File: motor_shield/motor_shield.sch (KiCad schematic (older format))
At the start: 23 parts, among them J1 MOTOR PWR, J2 Conn_01x04, J3 Conn_01x04, J4 Conn_01x04, J5 ARDUINO PWR, J6 RPI PWR, J7 Raspberry_Pi_2_3, U1 DRV8834_CARRIER, U10 SHARP_GP2Y0A21YK0F, U2 DRV8834_CARRIER, U3 DRV8834_CARRIER, U4 ARDUINO_MICRO, U5 SHARP_GP2Y0A21YK0F, U6 SHARP_GP2Y0A21YK0F, U7 SHARP_GP2Y0A21YK0F, U8 SHARP_GP2Y0A21YK0F, U9 SHARP_GP2Y0A21YK0F

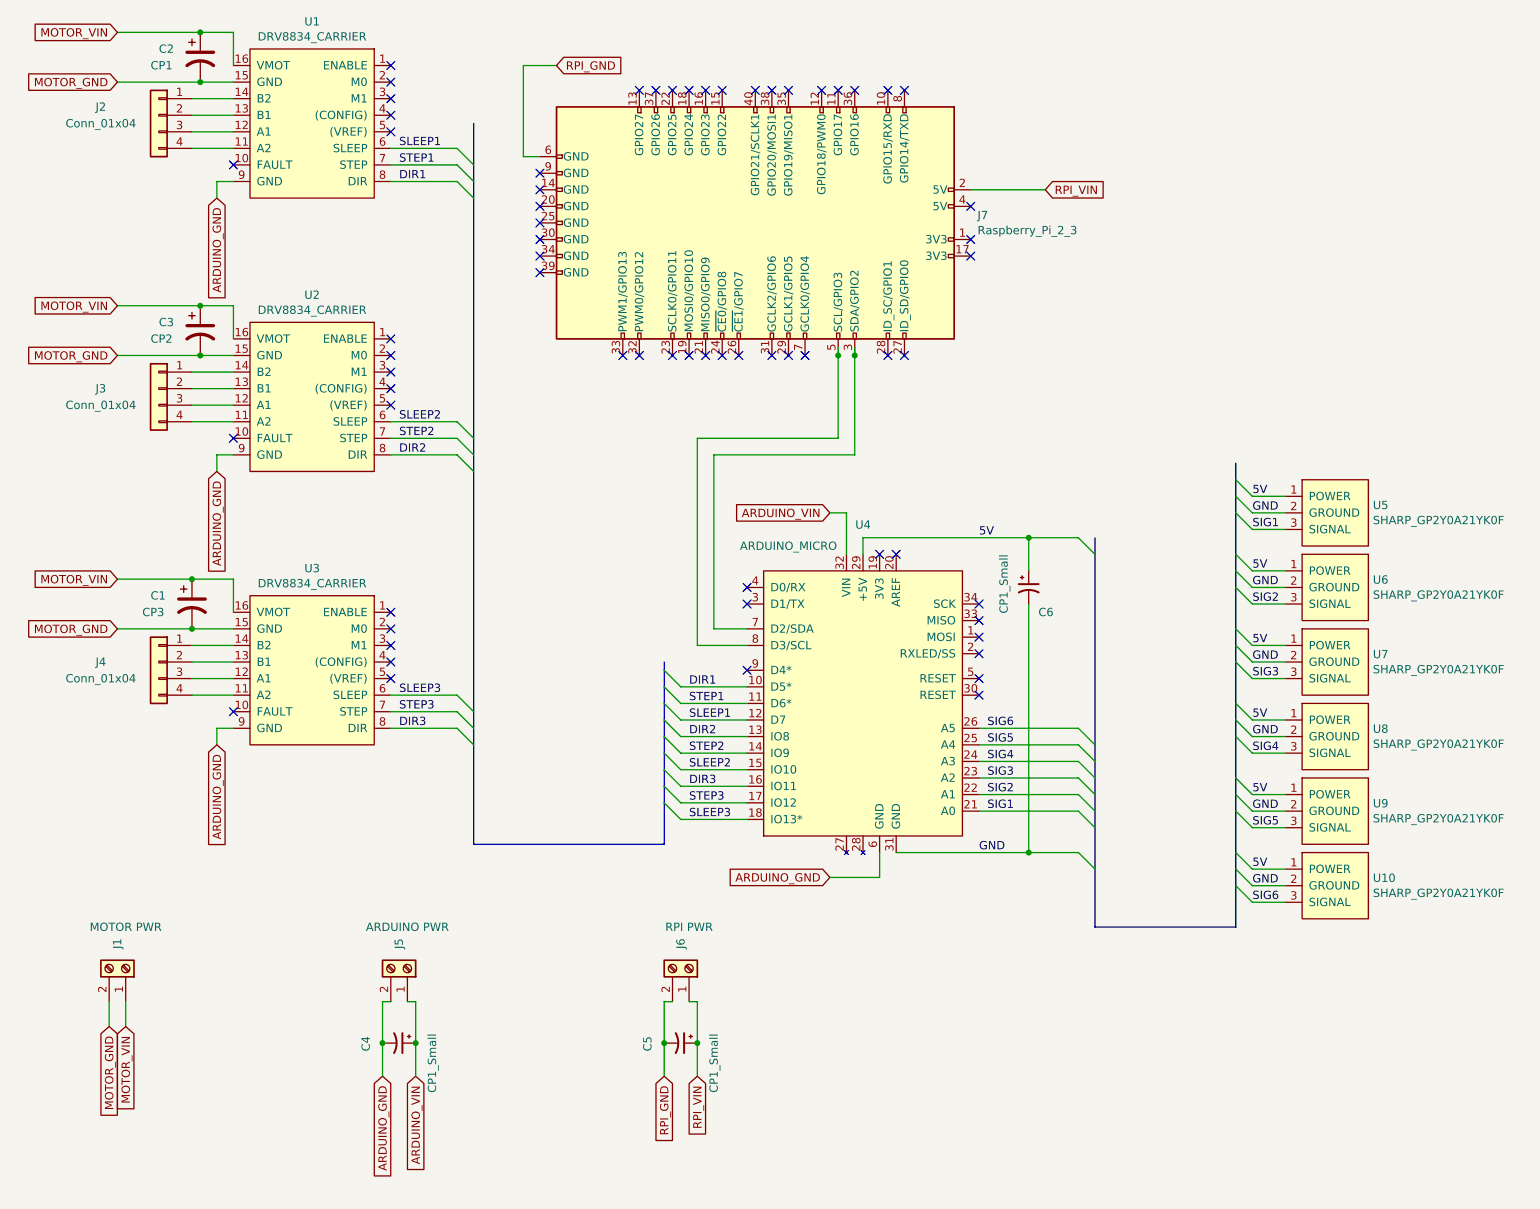
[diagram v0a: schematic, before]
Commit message: Finish circuit board design
off to oshpark!
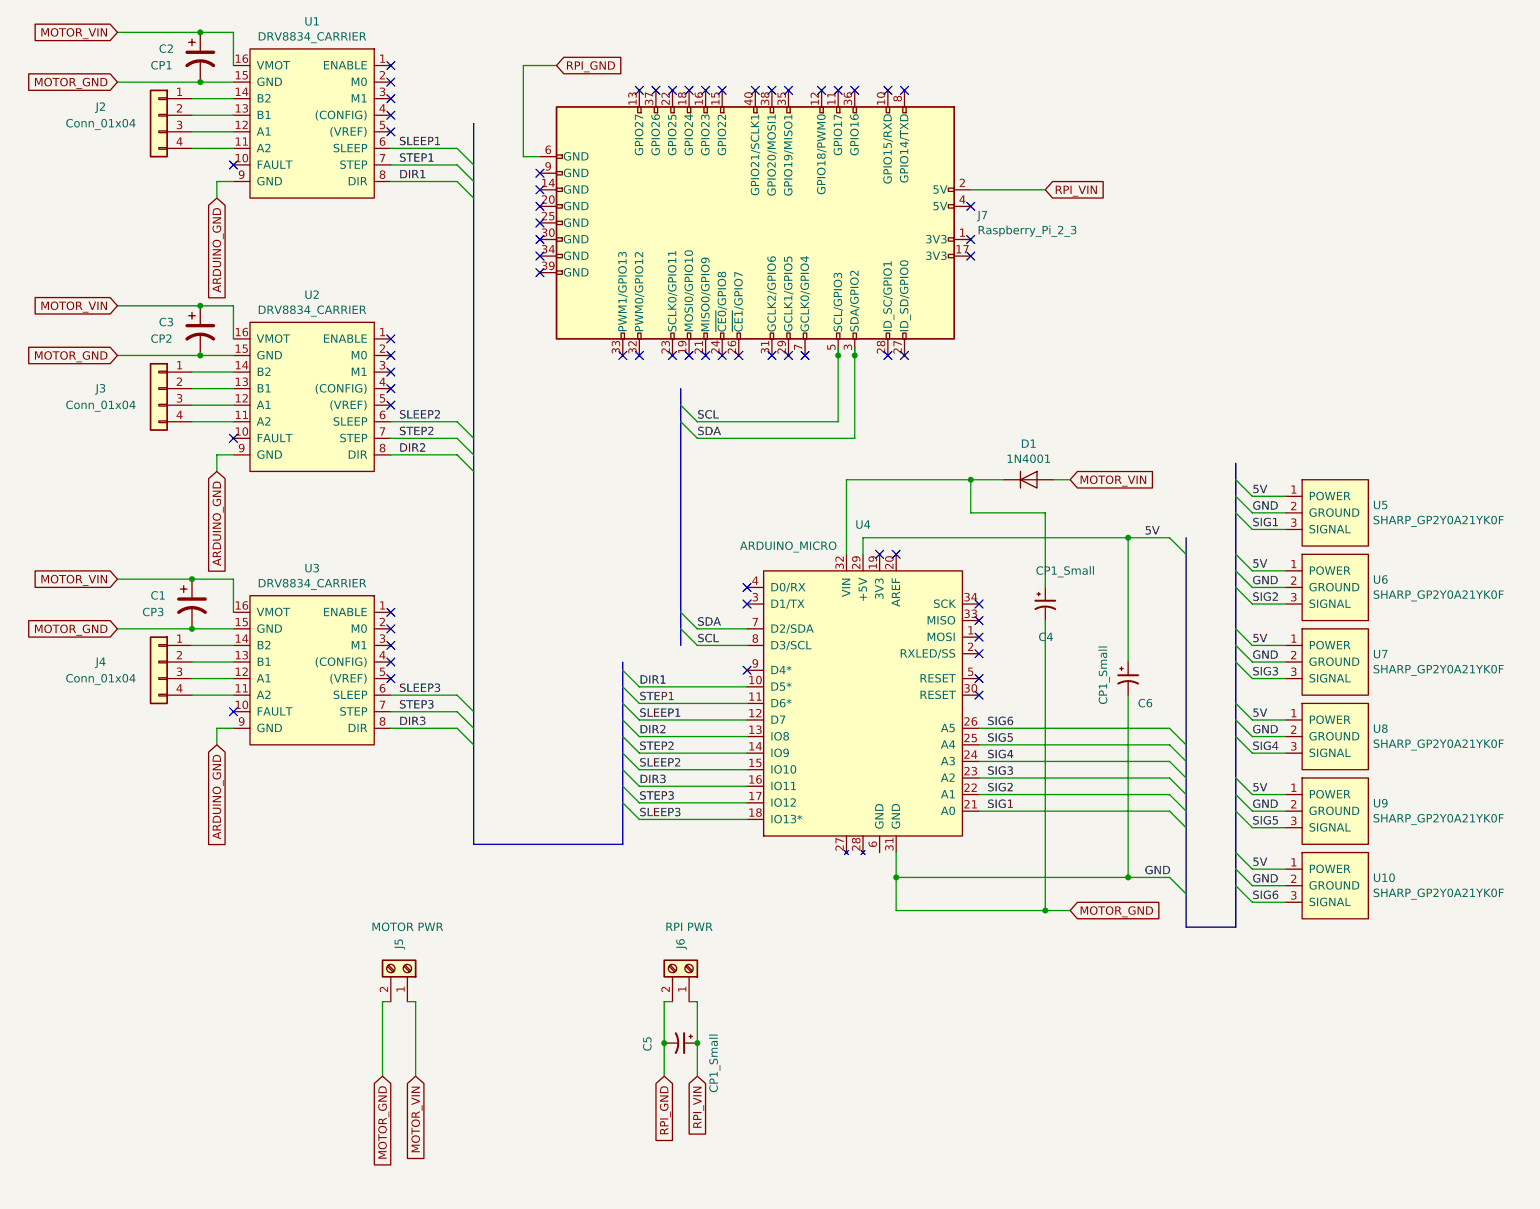
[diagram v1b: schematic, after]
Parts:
- removed J1: MOTOR PWR, CATPOO:TerminalBlock_Pololu-2_P5.00mm, symbol Connector:Screw_Terminal_01x02
- added D1: 1N4001, Diode_THT:D_DO-41_SOD81_P10.16mm_Horizontal, symbol Diode:1N4001
- J5: value ARDUINO PWR -> MOTOR PWR
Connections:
- net GND is gone; now on net MOTOR_GND: C6.2, U10.2 (GROUND), U4.31 (GND), U5.2 (GROUND), U6.2 (GROUND), U7.2 (GROUND), U8.2 (GROUND), U9.2 (GROUND)
- net ARDUINO_GND: no longer C4.2, J5.2 (Pin_2), U4.6 (GND)
- net MOTOR_GND: now also C4.2, J5.2 (Pin_2)
- net MOTOR_VIN: now also J5.1 (Pin_1), D1.2 (A)
- net SDA: now reaches J7.3 (SDA/GPIO2), U4.7 (D2/SDA)
- net SCL: now reaches J7.5 (SCL/GPIO3), U4.8 (D3/SCL)
- net ARDUINO_VIN: no longer names the net of C4.1, U4.32 (VIN)
- net ARDUINO_VIN: now also D1.1 (K); no longer J5.1 (Pin_1)
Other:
- moved on the sheet: C4, C6
